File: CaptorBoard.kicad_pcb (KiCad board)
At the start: 2 copper layers, 70 x 45 mm, 23 parts, among them J1 Conn_01x06, J2 Screw_Terminal_01x04, SW1 SKHHLVA010, SW2 SKHHLVA010, U1 WeMos_mini, U2 IRM-02-5, U3 MOC3041M, U4 MOC3041M, U5 DHT22

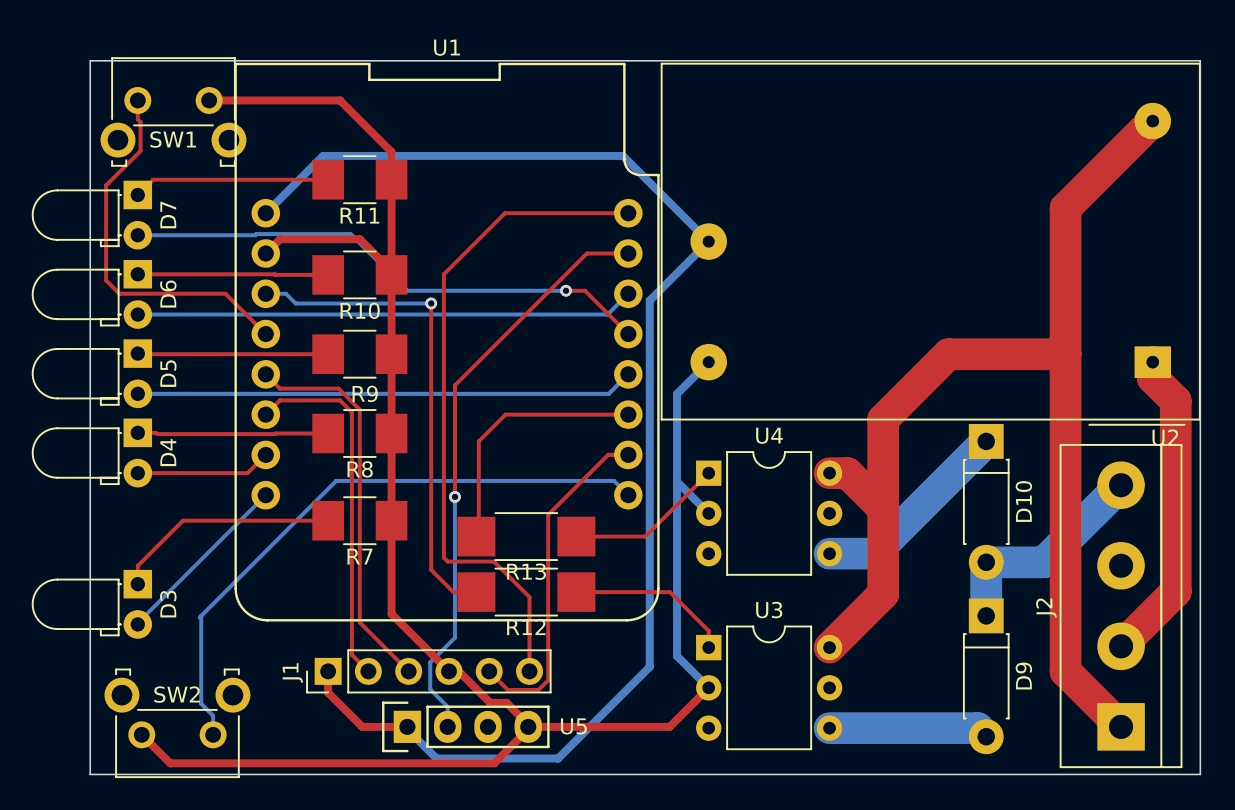
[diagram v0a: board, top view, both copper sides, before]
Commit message: Board final
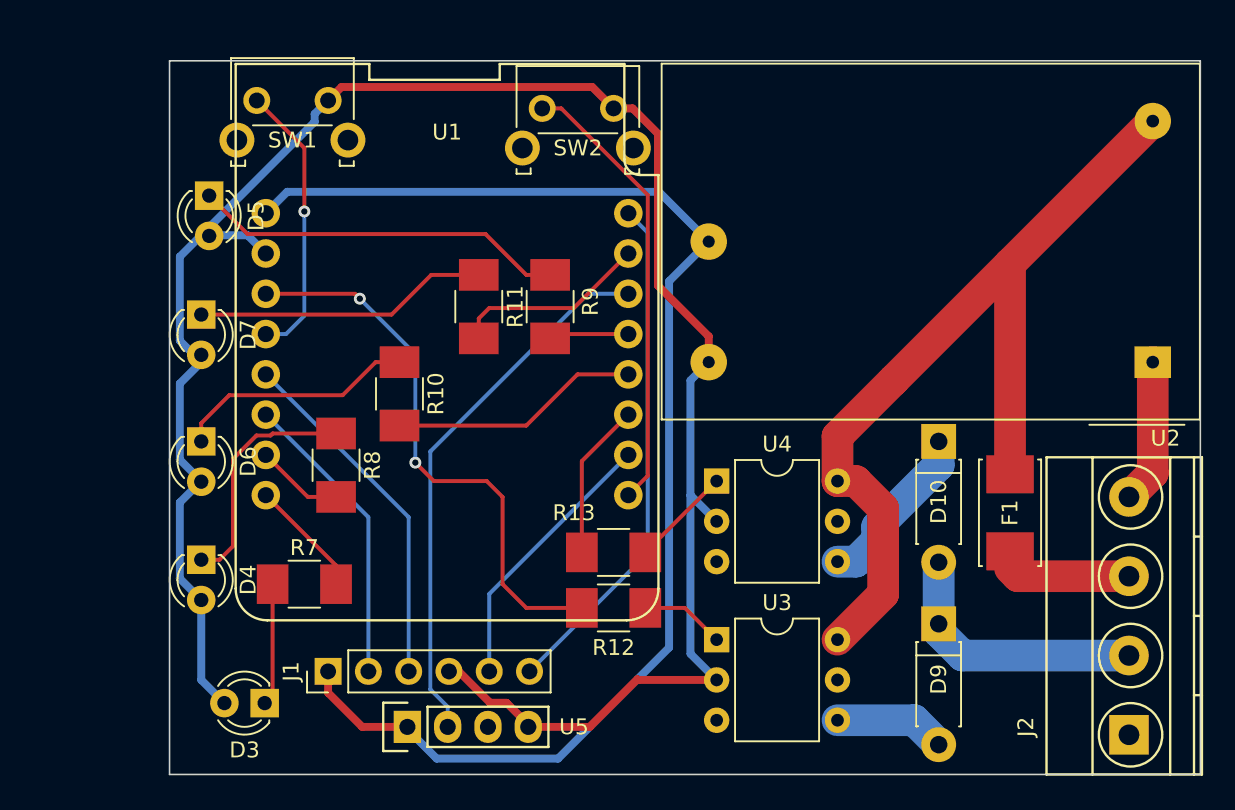
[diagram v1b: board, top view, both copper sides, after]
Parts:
- added F1: Fuse_Small, Fuse:Fuseholder_Littelfuse_Nano2_157x, F.Cu at (128.0, 83.5)
- D3, D4, D5, D6, D7: footprint LEDs:LED_D3.0mm_Horizontal_O1.27mm_Z2.0mm -> LEDs:LED_D3.0mm
- J2: value Screw_Terminal_01x04 -> MKDSN 1,5/ 4-5,08; footprint Connectors_Terminal_Blocks:TerminalBlock_bornier-4_P5.08mm -> TerminalBlocks_Phoenix:TerminalBlock_Phoenix_MKDS1.5-4pol
- R12, R13: footprint Resistors_SMD:R_2010_HandSoldering -> Resistors_SMD:R_1210_HandSoldering
- U3, U4: value MOC3041M -> MOC3040X
- moved SW2 44.6 mm to (98.5, 58.0), turned to 0 degrees
- moved R9 12.4 mm to (99.0, 70.5), turned to 270 degrees
- moved D6 11.3 mm to (77.0, 79.0)
- moved D3 11.0 mm to (81.0, 95.5), turned to 180 degrees
- moved R11 11.0 mm to (94.5, 70.5), turned to 270 degrees
- moved D5 10.9 mm to (77.5, 63.5)
- moved D4 8.94 mm to (77.0, 86.5)
- moved D7 8.54 mm to (77.0, 71.0)
- moved R10 7.91 mm to (89.5, 76.0), turned to 270 degrees
- moved SW1 7.50 mm to (80.5, 57.5)
- moved R12 5.59 mm to (103.0, 89.5)
- moved R13 5.59 mm to (103.0, 86.0)
- moved R7 5.32 mm to (83.5, 88.0), turned to 0 degrees
- moved D9 3.04 mm to (123.5, 90.5)
- moved D10 3.00 mm to (123.5, 79.0)
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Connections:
- D10 pad 2: /Pilote -> /CMD2
- D3 pad 2: /POWER -> GND
- D4 pad 2: /CONF -> GND
- D5 pad 2: /ECO -> GND
- D6 pad 2: /CONF-1°C -> GND
- D7 pad 2: /CONF-2°C -> GND
- D9 pad 1: /Pilote -> /CMD2
- J2 pad 1: /Phase -> (no net)
- J2 pad 2: /Neutre -> /CMD2
- J2 pad 3: (no net) -> Net-(F1-Pad2)
- J2 pad 4: /Pilote -> /Neutre
- R10 pad 1: GND -> Net-(D6-Pad1)
- R10 pad 2: Net-(D6-Pad1) -> /CONF-1°C
- R11 pad 1: GND -> Net-(D7-Pad1)
- R11 pad 2: Net-(D7-Pad1) -> /CONF-2°C
- R7 pad 1: GND -> Net-(D3-Pad1)
- R7 pad 2: Net-(D3-Pad1) -> /POWER
- R8 pad 1: GND -> Net-(D4-Pad1)
- R8 pad 2: Net-(D4-Pad1) -> /CONF
- R9 pad 1: GND -> Net-(D5-Pad1)
- R9 pad 2: Net-(D5-Pad1) -> /ECO
- U1 pad 12: /ECO -> /CONF-1°C
- U1 pad 13: /CONF-2°C -> /ECO
- U1 pad 14: /CONF-1°C -> /CAPTOR
- U1 pad 15: /CAPTOR -> /CONF-2°C
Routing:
- net /ECO: track 31.4 -> 5.04 mm
- net /CONF-2°C: track 33.6 -> 12.4 mm, vias 1 -> 0
- net /Phase: track 75.2 -> 57.4 mm
- net /CMD2: track 0.00 -> 17.0 mm
- net /Pilote: track 16.4 -> 0.00 mm
- net /CONF-1°C: track 31.5 -> 15.8 mm
- net Net-(D5-Pad1): track 12.0 -> 23.6 mm
- net /Neutre: track 19.9 -> 9.12 mm
- net /RESET: track 38.8 -> 28.4 mm
- net +3V3: track 42.2 -> 32.5 mm
- net Net-(F1-Pad2): track 0.00 -> 7.71 mm
- net /PILOT_2: track 16.2 -> 9.65 mm
- net Net-(D3-Pad1): track 14.3 -> 7.81 mm
- net Net-(D7-Pad1): track 12.4 -> 18.5 mm
- net /SELECT: track 23.8 -> 17.7 mm, vias 0 -> 1
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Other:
- board size 70 x 45 mm -> 65 x 45 mm
- net class Sector: clearance 0.5 -> 0.7
- board text added: "1 - +5V 2 - CAPTEUR 3 - NC 4 - GND"
- board text added: "1 - Terre 2 - Pilote 3 - Phase 4 - Neutre"
- board text removed: "Neutre"
- board text removed: "Phase"
- board text removed: "Pilote"
- board text removed: "Terre"
